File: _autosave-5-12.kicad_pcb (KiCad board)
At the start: 2 copper layers, 266.7 x 95.2 mm, 136 parts, among them SW1 SW_Push, U1 ATmega32U4-AU, Y1 16MHz

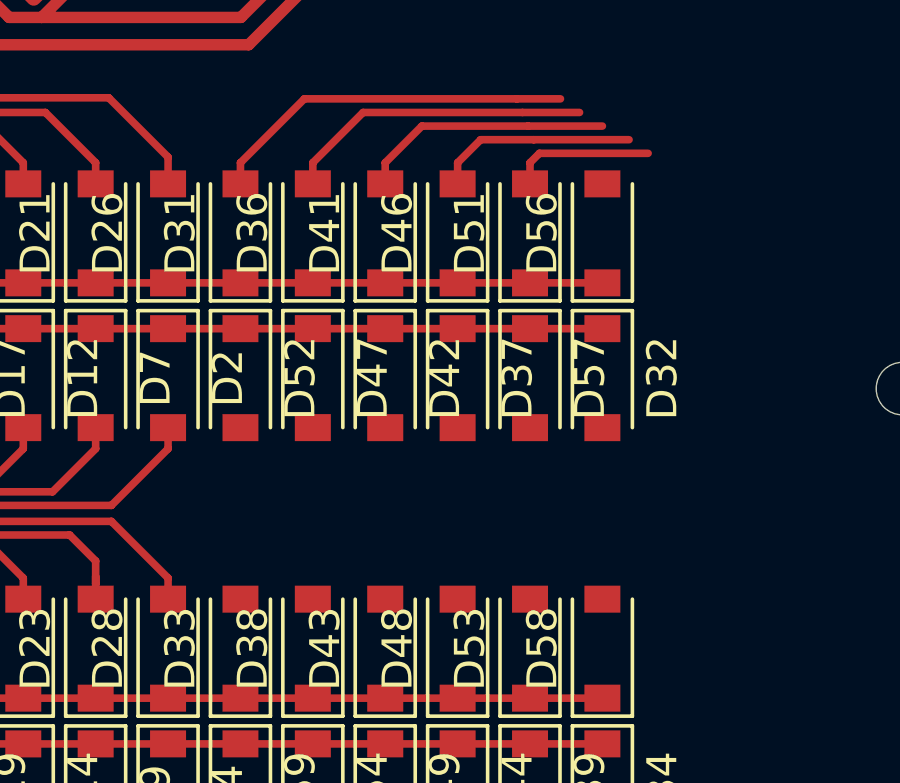
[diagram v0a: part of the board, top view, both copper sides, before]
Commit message: morning transfer
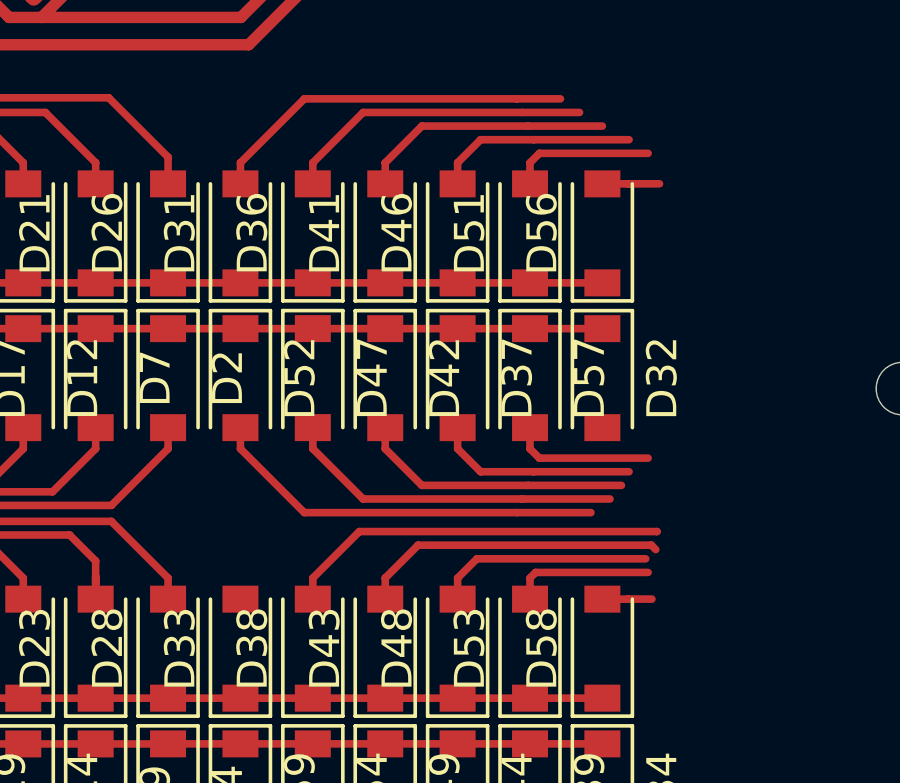
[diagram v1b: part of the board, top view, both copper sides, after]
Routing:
- net Net-(D52-Pad2): track 0.00 -> 13.3 mm
- net Net-(D38-Pad2): track 0.00 -> 12.8 mm
- net Net-(D47-Pad2): track 0.00 -> 11.3 mm
- net Net-(D43-Pad2): track 0.00 -> 10.2 mm
- net Net-(D42-Pad2): track 0.00 -> 9.08 mm
- net Net-(D48-Pad2): track 0.00 -> 7.24 mm
- net Net-(D37-Pad2): track 0.00 -> 6.74 mm
- net Net-(D57-Pad2): track 0.00 -> 4.77 mm
- net Net-(D53-Pad2): track 0.00 -> 4.72 mm
- net Net-(D56-Pad2): track 0.00 -> 1.91 mm
- net Net-(D58-Pad2): track 0.00 -> 1.65 mm
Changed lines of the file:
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@@
     (thickness 1.6)
     (drawings 8)
-    (tracks 621)
+    (tracks 660)
     (zones 0)
     (modules 136)
@@
   (segment (start 150.77303 107.47697) (end 156.086829 107.47697) (width 0.254) (layer F.Cu) (net 46))
   (segment (start 156.086829 107.47697) (end 157.988 107.47697) (width 0.254) (layer F.Cu) (net 46))
+  (segment (start 153.924 118.687) (end 154.69001 119.45301) (width 0.254) (layer F.Cu) (net 47))
+  (segment (start 153.924 117.983) (end 153.924 118.687) (width 0.254) (layer F.Cu) (net 47))
+  (segment (start 154.69001 119.45301) (end 156.460943 119.45301) (width 0.254) (layer F.Cu) (net 47))
+  (segment (start 156.460943 119.45301) (end 159.639 119.45301) (width 0.254) (layer F.Cu) (net 47))
+  (segment (start 150.64703 121.44697) (end 160.570037 121.44697) (width 0.254) (layer F.Cu) (net 48))
+  (segment (start 149.098 123.7) (end 149.098 122.996) (width 0.254) (layer F.Cu) (net 48))
+  (segment (start 149.098 122.996) (end 150.64703 121.44697) (width 0.254) (layer F.Cu) (net 48))
+  (segment (start 160.570037 121.44697) (end 160.570037 121.446971) (width 0.254) (layer F.Cu) (net 48))
   (segment (start 195.42125 149.70125) (end 188.24575 149.70125) (width 0.254) (layer F.Cu) (net 50))
   (segment (start 188.24575 149.70125) (end 185.547 152.4) (width 0.254) (layer F.Cu) (net 50))
@@
   (segment (start 152.73302 107.93098) (end 156.274886 107.93098) (width 0.254) (layer F.Cu) (net 51))
   (segment (start 156.274886 107.93098) (end 158.75 107.93098) (width 0.254) (layer F.Cu) (net 51))
+  (segment (start 151.511 118.687) (end 152.73102 119.90702) (width 0.254) (layer F.Cu) (net 52))
+  (segment (start 151.511 117.983) (end 151.511 118.687) (width 0.254) (layer F.Cu) (net 52))
+  (segment (start 152.73102 119.90702) (end 156.272886 119.90702) (width 0.254) (layer F.Cu) (net 52))
+  (segment (start 156.272886 119.90702) (end 159.385 119.90702) (width 0.254) (layer F.Cu) (net 52))
+  (segment (start 152.60602 121.90098) (end 160.38198 121.90098) (width 0.254) (layer F.Cu) (net 53))
+  (segment (start 151.511 123.7) (end 151.511 122.996) (width 0.254) (layer F.Cu) (net 53))
+  (segment (start 151.511 122.996) (end 152.60602 121.90098) (width 0.254) (layer F.Cu) (net 53))
+  (segment (start 160.38198 121.90098) (end 160.528 122.047) (width 0.254) (layer F.Cu) (net 53))
   (segment (start 196.723 147.574) (end 198.85025 149.70125) (width 0.254) (layer F.Cu) (net 55))
   (segment (start 194.31 147.574) (end 196.723 147.574) (width 0.254) (layer F.Cu) (net 55))
@@
   (segment (start 154.69201 108.38499) (end 156.462943 108.38499) (width 0.254) (layer F.Cu) (net 56))
   (segment (start 156.462943 108.38499) (end 159.639 108.38499) (width 0.254) (layer F.Cu) (net 56))
+  (segment (start 149.098 118.685) (end 150.77403 120.36103) (width 0.254) (layer F.Cu) (net 57))
+  (segment (start 149.098 117.981) (end 149.098 118.685) (width 0.254) (layer F.Cu) (net 57))
+  (segment (start 150.77403 120.36103) (end 156.084829 120.36103) (width 0.254) (layer F.Cu) (net 57))
+  (segment (start 156.084829 120.36103) (end 159.004 120.36103) (width 0.254) (layer F.Cu) (net 57))
+  (segment (start 153.924 123.7) (end 153.924 122.996) (width 0.254) (layer F.Cu) (net 58))
+  (segment (start 153.924 122.996) (end 154.56501 122.35499) (width 0.254) (layer F.Cu) (net 58))
+  (segment (start 154.56501 122.35499) (end 160.193924 122.35499) (width 0.254) (layer F.Cu) (net 58))
   (segment (start 153.924 142.494) (end 153.924 139.446) (width 0.254) (layer F.Cu) (net 60))
   (segment (start 158.242 146.685) (end 153.924 142.494) (width 0.254) (layer F.Cu) (net 60))
@@
   (segment (start 156.337 109.857) (end 156.337 109.153) (width 0.254) (layer F.Cu) (net 61))
   (segment (start 156.651 108.839) (end 160.274 108.839) (width 0.254) (layer F.Cu) (net 61))
+  (segment (start 146.685 118.687) (end 148.81304 120.81504) (width 0.254) (layer F.Cu) (net 62))
+  (segment (start 146.685 117.983) (end 146.685 118.687) (width 0.254) (layer F.Cu) (net 62))
+  (segment (start 148.81304 120.81504) (end 155.896772 120.81504) (width 0.254) (layer F.Cu) (net 62))
+  (segment (start 155.896772 120.81504) (end 158.369 120.81504) (width 0.254) (layer F.Cu) (net 62))
+  (segment (start 156.337 122.996) (end 156.524 122.809) (width 0.254) (layer F.Cu) (net 63))
+  (segment (start 156.337 123.7) (end 156.337 122.996) (width 0.254) (layer F.Cu) (net 63))
+  (segment (start 156.524 122.809) (end 160.274 122.809) (width 0.254) (layer F.Cu) (net 63))
   (segment (start 156.337 139.446) (end 156.337 143.256) (width 0.254) (layer F.Cu) (net 65))
   (segment (start 156.337 143.256) (end 158.623 145.542) (width 0.254) (layer F.Cu) (net 65))
@@
   (segment (start 212.852 146.939) (end 212.09 147.701) (width 0.254) (layer F.Cu) (net 65))
   (segment (start 212.09 147.701) (end 201.422 147.701) (width 0.254) (layer F.Cu) (net 65))
+  (segment (start 159.604 109.857) (end 159.606 109.855) (width 0.254) (layer F.Cu) (net 66))
+  (segment (start 158.75 109.857) (end 159.604 109.857) (width 0.254) (layer F.Cu) (net 66))
+  (segment (start 159.606 109.855) (end 160.655 109.855) (width 0.254) (layer F.Cu) (net 66))
+  (segment (start 156.337 118.687) (end 156.649 118.999) (width 0.254) (layer F.Cu) (net 67))
+  (segment (start 156.337 117.983) (end 156.337 118.687) (width 0.254) (layer F.Cu) (net 67))
+  (segment (start 156.649 118.999) (end 160.274 118.999) (width 0.254) (layer F.Cu) (net 67))
+  (segment (start 159.604 123.7) (end 159.606 123.698) (width 0.254) (layer F.Cu) (net 68))
+  (segment (start 158.75 123.7) (end 159.604 123.7) (width 0.254) (layer F.Cu) (net 68))
+  (segment (start 159.606 123.698) (end 160.401 123.698) (width 0.254) (layer F.Cu) (net 68))
   (segment (start 158.75 143.383) (end 158.75 139.446) (width 0.254) (layer F.Cu) (net 70))
   (segment (start 172.974 142.875) (end 170.942 144.78) (width 0.254) (layer F.Cu) (net 70))
